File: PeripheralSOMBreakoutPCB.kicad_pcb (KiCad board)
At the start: 2 copper layers, 32 x 57.2 mm, 11 parts, among them J1 Conn_01x02, J2 Conn_01x02, J3 Conn_01x02, J4 Conn_01x02, J5 Conn_01x04, J6 Conn_01x04, J7 Conn_01x01, J8 Conn_01x01

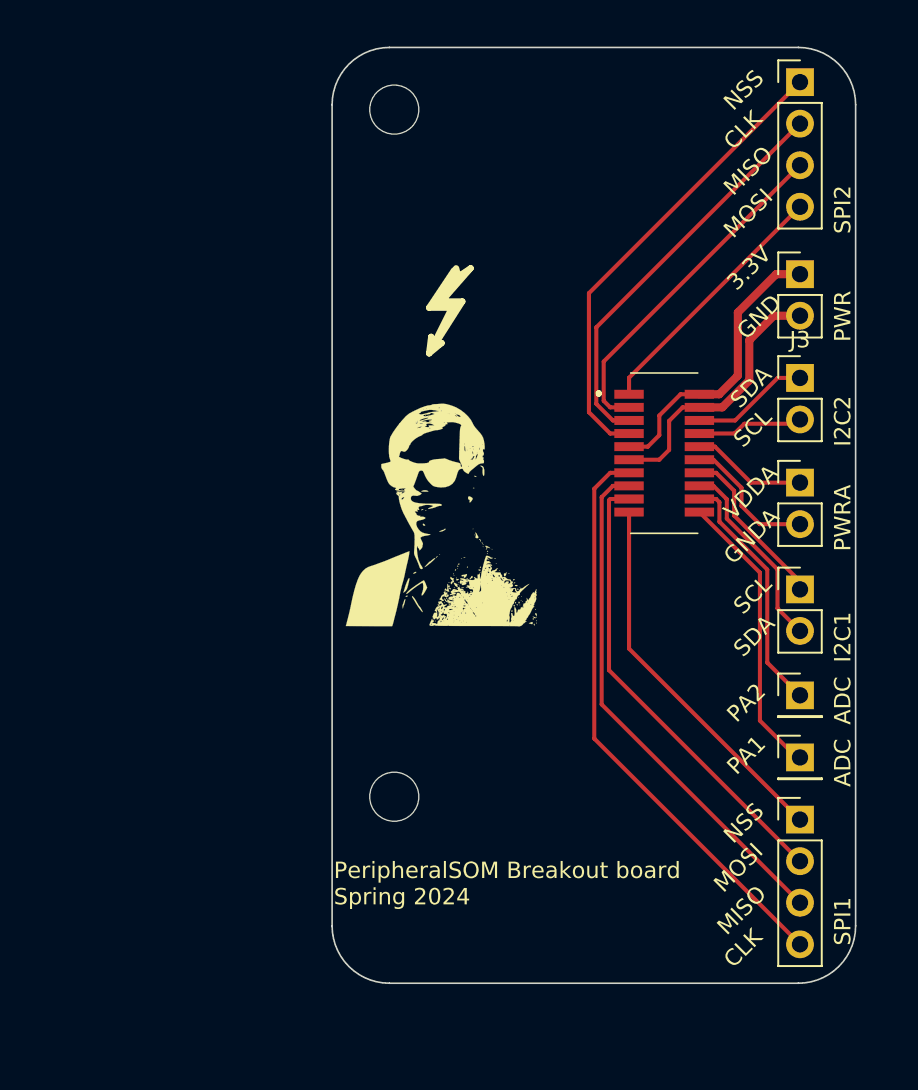
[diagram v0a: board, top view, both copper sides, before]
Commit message: board
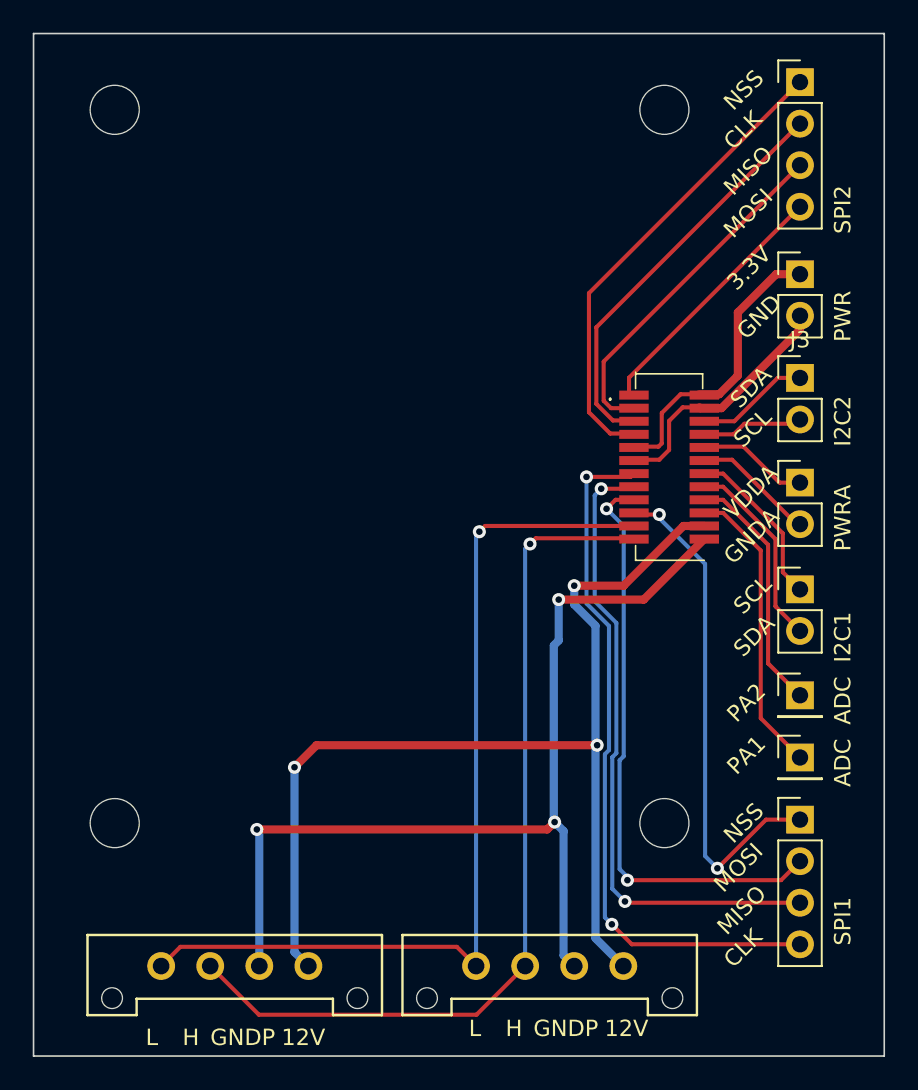
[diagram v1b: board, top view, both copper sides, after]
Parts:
- removed G***: LOGO, UTSVT_Special:Hallock_Image_Tiny
- removed REF**: Symbol_HighVoltage_Small, UTSVT_Special:Symbol_HighVoltage_Small
- added J10: CANConnector, UTSVT_Connectors:Molex_MicroFit3.0_1x4xP3.00mm_PolarizingPeg_Vertical, F.Cu at (152.6, 129.6)
- added J9: CANConnector, UTSVT_Connectors:Molex_MicroFit3.0_1x4xP3.00mm_PolarizingPeg_Vertical, F.Cu at (133.3, 129.6)
- U1: value ~ -> PeripheralSOM
- moved U1 3.38 mm to (137.1, 95.8)
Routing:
- net +12V: track 0.00 -> 65.5 mm, vias 0 -> 3
- net GNDPWR: track 0.00 -> 60.3 mm, vias 0 -> 3
- net /CAN_L: track 0.00 -> 56.5 mm, vias 0 -> 1
- net /CAN_H: track 0.00 -> 54.2 mm, vias 0 -> 1
- net /SPI1_MOSI: track 28.2 -> 36.4 mm, vias 0 -> 2
- net /SPI1_NSS: track 23.1 -> 31.0 mm, vias 0 -> 2
- net /SPI1_CLK: track 35.6 -> 43.2 mm, vias 0 -> 2
- net /SPI1_MISO: track 31.8 -> 39.1 mm, vias 0 -> 2
- net GND: track 16.6 -> 15.7 mm
- net GNDA: track 8.43 -> 7.78 mm
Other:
- board size 32 x 57.2 mm -> 52 x 62.5 mm
- board text added: "12V"
- board text added: "GNDP"
- board text added: "H"
- board text added: "L"
- board text removed: "PeripheralSOM Breakout board Spring 2024"
